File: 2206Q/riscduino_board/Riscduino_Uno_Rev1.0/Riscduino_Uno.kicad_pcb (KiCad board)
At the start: 2 copper layers, 68.8 x 53.6 mm, 80 parts, among them J1 USB_B_Micro, J10 Conn_01x01, J11 Conn_01x01, J2 ISP, J3 Conn_01x08_Pin, J4 Conn_01x06_Pin, J5 Conn_01x08_Pin, J6 Conn_01x10_Pin, J7 Conn_02x04_Odd_Even, J8 Conn_01x01, J9 Conn_01x01, SW1 4Pin Round Button SPST Straig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, U1 LM1117S-ADJ, U2 LM1117MP-3.3, U3 Riscduino, U4 CP2102N-Axx-xQFN28, U5 W25Q32JVSS, U6 W25Q32JVSS, U7 23LC1024-I/P, U8 MAX1232ESA+T, X1 ASE-10.000MHZ-LC-T

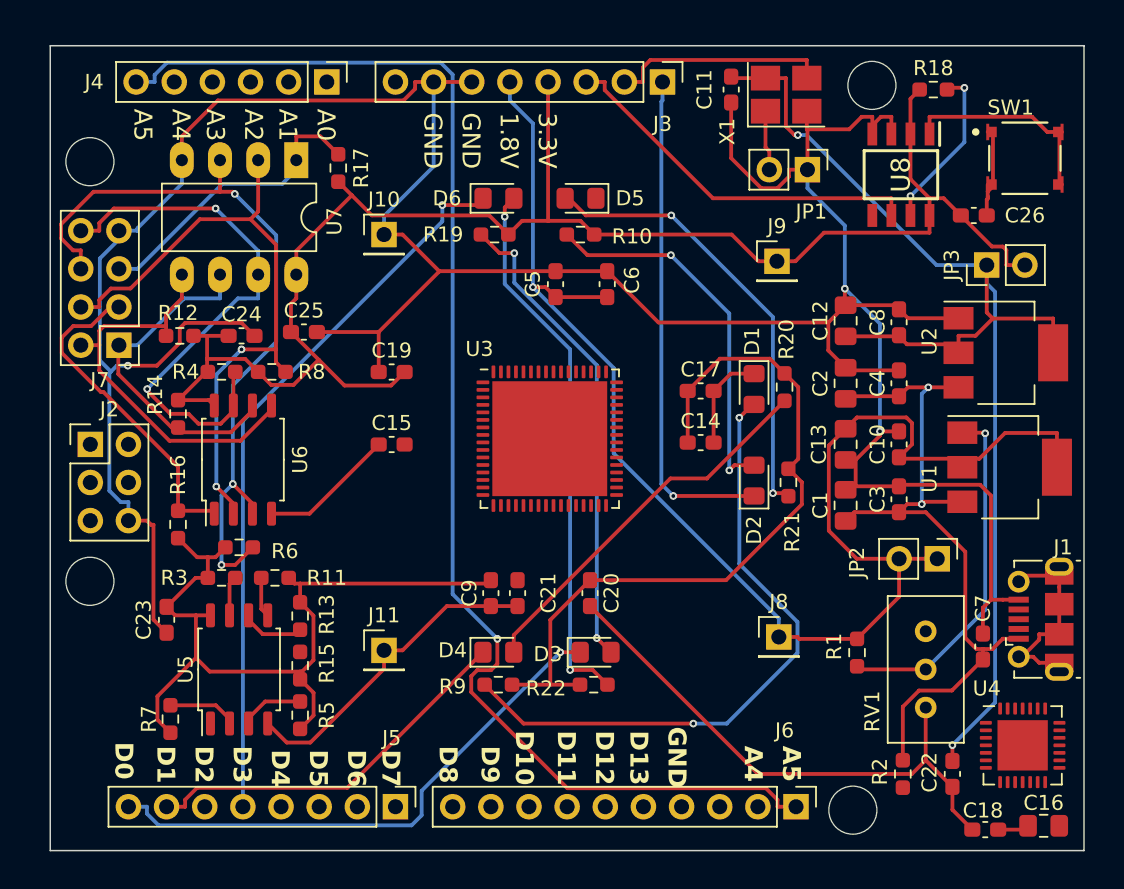
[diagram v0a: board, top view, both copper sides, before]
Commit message: 1.0.3 Update
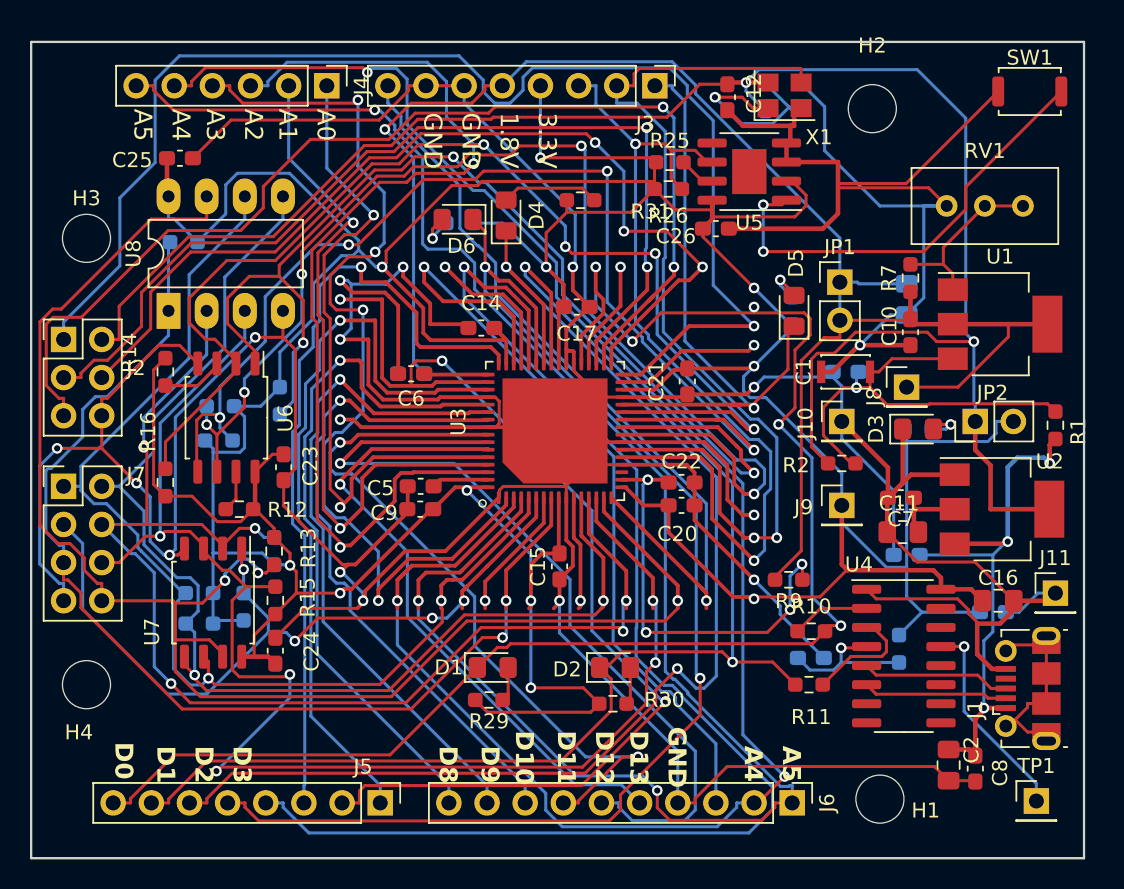
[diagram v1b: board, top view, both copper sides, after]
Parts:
- removed JP3: Jumper_2, Connector_PinHeader_2.54mm:PinHeader_1x02_P2.54mm_Vertical
- removed REF**: Riscduino_UNO_R0_WithMountingHoles, Riscduino.Library:Riscduino_UNO_R0_WithMountingHoles
- added H1: MountingHole, MountingHole:MountingHole_3.2mm_M3, F.Cu at (126.2, 99.8)
- added H2: MountingHole, MountingHole:MountingHole_3.2mm_M3, F.Cu at (125.7, 53.8)
- added H3: MountingHole, MountingHole:MountingHole_3.2mm_M3, F.Cu at (73.4, 62.5)
- added H4: MountingHole, MountingHole:MountingHole_3.2mm_M3, F.Cu at (73.4, 92.2)
- added R23: 10K, Resistor_SMD:R_0603_1608Metric_Pad0.98x0.95mm_HandSolder, B.Cu at (83.9, 87.0)
- added R24: 10K, Resistor_SMD:R_0603_1608Metric_Pad0.98x0.95mm_HandSolder, B.Cu at (79.9, 62.7)
- added R25: 10K, Resistor_SMD:R_0603_1608Metric_Pad0.98x0.95mm_HandSolder, F.Cu at (112.2, 57.4)
- added R26: 10K, Resistor_SMD:R_0603_1608Metric_Pad0.98x0.95mm_HandSolder, F.Cu at (112.1, 59.2)
- added R27: 470 Ohm, Resistor_SMD:R_0603_1608Metric_Pad0.98x0.95mm_HandSolder, B.Cu at (128.8, 75.2)
- added R28: 470 Ohm, Resistor_SMD:R_0603_1608Metric_Pad0.98x0.95mm_HandSolder, B.Cu at (120.4, 67.3)
- added R29: 470 Ohm, Resistor_SMD:R_0603_1608Metric_Pad0.98x0.95mm_HandSolder, F.Cu at (100.2, 93.2)
- added R30: 470 Ohm, Resistor_SMD:R_0603_1608Metric_Pad0.98x0.95mm_HandSolder, F.Cu at (108.5, 93.5)
- added R31: 470 Ohm, Resistor_SMD:R_0603_1608Metric_Pad0.98x0.95mm_HandSolder, F.Cu at (106.3, 59.9)
- added R32: 470 Ohm, Resistor_SMD:R_0603_1608Metric_Pad0.98x0.95mm_HandSolder, B.Cu at (98.3, 61.5)
- added TP1: TestPoint, Connector_PinHeader_2.54mm:PinHeader_1x01_P2.54mm_Vertical, F.Cu at (136.7, 99.9)
- C1: footprint Capacitor_SMD:C_0805_2012Metric_Pad1.18x1.45mm_HandSolder -> Button_Switch_SMD:SW_SPST_CK_KXT3
- C11: value 0.1uF -> 22uF; footprint Capacitor_SMD:C_0603_1608Metric_Pad1.08x0.95mm_HandSolder -> Capacitor_SMD:C_0805_2012Metric_Pad1.18x1.45mm_HandSolder
- C12: value 22uF -> 0.1uF; footprint Capacitor_SMD:C_0805_2012Metric_Pad1.18x1.45mm_HandSolder -> Capacitor_SMD:C_0603_1608Metric_Pad1.08x0.95mm_HandSolder
- C13, C18, C3, C4, R17, R18: moved to B.Cu
- C19: value 0.1uf -> 0.1uF; moved to B.Cu
- C22: value 0.1uF -> 0.1uf
- D1: value RED LED -> BLUE LED
- D3: value BLUE LED -> RED LED
- JP1: value Jumper_2_Open -> Jumper_2
- R1: value 470 Ohm -> DNI
- R10, R9: value 470 Ohm -> 0E
- R11, R2: value 10K -> 0E
- R19, R20, R21, R22: value 470 Ohm -> 10K; moved to B.Cu
- R3, R4, R8: value 10K -> 0E; moved to B.Cu
- R5, R6: value 10K -> DNI; moved to B.Cu
- R7: value 10K -> 470 Ohm
- SW1: footprint Switch_E-Switch_TL3315NF250Q:E-Switch-TL3315NF250Q-0-0-0 -> Button_Switch_SMD:SW_Push_SPST_NO_Alps_SKRK
- U3: footprint Package_DFN_QFN:QFN-64-1EP_9x9mm_P0.5mm_EP7.65x7.65mm -> Package_DFN_QFN:RISCDUINO_QFN-64-1EP_9x9mm_P0.5mm_EP7.65x7.65mm_NEW
- U4: value CP2102N-Axx-xQFN28 -> CH340C; footprint Package_DFN_QFN:QFN-28-1EP_5x5mm_P0.5mm_EP3.35x3.35mm -> Package_SO:SOIC-16_3.9x9.9mm_P1.27mm
- U5: value W25Q32JVSS -> MAX1232ESA+T; footprint Package_SO:SOIC-8_5.23x5.23mm_P1.27mm -> Package_SO:SOIC-8-1EP_3.9x4.9mm_P1.27mm_EP2.29x3mm
- U7: value 23LC1024-I/P -> W25Q32JVSS; footprint Package_DIP:DIP-8_W7.62mm_LongPads -> Package_SO:SOIC-8_5.23x5.23mm_P1.27mm
- U8: value MAX1232ESA+T -> 23LC1024-I/P; footprint MAX1232ESA+T:SOIC127P600X175-8N -> Package_DIP:DIP-8_W7.62mm_LongPads
- X1: footprint Oscillator:Oscillator_SMD_Abracon_ASE-4Pin_3.2x2.5mm_HandSoldering -> Crystal:Crystal_SMD_Abracon_ABM8G-4Pin_3.2x2.5mm
- moved R7 57.4 mm to (128.3, 65.1)
- moved R18 53.0 mm to (82.2, 75.9)
- moved R5 51.5 mm to (118.6, 53.1)
- moved U8 49.6 mm to (78.9, 67.3), turned to 90 degrees
- moved R6 47.9 mm to (120.9, 53.0), turned to 90 degrees
- moved U5 47.5 mm to (117.5, 58.0), turned to 180 degrees
- moved R8 45.6 mm to (127.5, 89.8), turned to 90 degrees
- moved J11 44.9 mm to (137.9, 86.1)
- moved R21 39.9 mm to (80.9, 86.1), turned to 180 degrees
- moved R20 37.6 mm to (82.3, 73.7), turned to 180 degrees
- moved R11 36.3 mm to (121.5, 92.2)
- moved C19 33.8 mm to (121.6, 90.4), turned to 180 degrees
- moved J10 32.9 mm to (123.7, 74.7)
- moved R19 32.5 mm to (80.9, 88.1), turned to 180 degrees
- moved C11 31.6 mm to (127.8, 82.0), turned to 180 degrees
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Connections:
- C1 pad 1: +5V -> Net-(U1-VI)
- C16 pad 1: +5V -> +3.3V
- C18 pad 1: +5V -> +3.3V
- C19 pad 2: +3.3V -> Net-(U4-V3)
- C20 pad 1: +3.3V -> GND
- C20 pad 2: GND -> +3.3V
- C21 pad 1: GND -> +3.3V
- C21 pad 2: +1V8 -> GND
- C22 pad 1: +3.3VP -> GND
- C22 pad 2: GND -> /vccd0
- C3 pad 1: +5V -> Net-(U1-VI)
- C5 pad 1: GND -> /vccd2
- C5 pad 2: +1V8 -> GND
- C6 pad 2: +1V8 -> /vccd1
- C7 pad 1: +5V -> +3.3VP
- C8 pad 1: +3.3VP -> +5V
- D1 pad 1: GND -> ardunio_d0
- D2 pad 1: gpio -> ardunio_d1
- D3 pad 1: ardunio_d0 -> GND
- D4 pad 1: ardunio_d1 -> ardunio_d2
- D5 pad 1: ardunio_d2 -> gpio
- JP1 pad 1: GND -> +1V8
- JP1 pad 2: Net-(JP1-B) -> +1V8
- JP2 pad 1: +1V8 -> +3.3VP
- JP2 pad 2: +1V8 -> +3.3V
- R1 pad 1: +1V8 -> +5V
- R1 pad 2: Net-(U1-ADJ) -> Net-(U1-VI)
- R10 pad 1: Net-(D2-A) -> Net-(U4-TXD)
- R10 pad 2: +3.3V -> ardunio_d0
- R11 pad 1: +3.3V -> Net-(U4-RXD)
- R11 pad 2: CARAVEL_FLASH_IO0 -> ardunio_d1
- R12 pad 2: USER_FLASH_IO0 -> CARAVEL_FLASH_IO3
- R13 pad 2: CARAVEL_FLASH_SCK -> USER_FLASH_IO3
- R14 pad 2: USER_FLASH_SCK -> CARAVEL_FLASH_IO2
- R15 pad 2: CARAVEL_FLASH_SSN -> USER_FLASH_IO2
- R16 pad 2: USER_FLASH_SSN -> CARAVEL_FLASH_IO1
- R17 pad 2: USER_SRAM_SSN -> USER_FLASH_IO1
- R18 pad 2: Net-(U8-~{ST}) -> CARAVEL_FLASH_IO0
- R19 pad 1: Net-(D3-A) -> +3.3V
- R19 pad 2: +3.3V -> USER_FLASH_IO0
- R2 pad 1: +5V -> +3.3VP
- R2 pad 2: Net-(U4-~{RST}) -> Net-(U1-VI)
- R20 pad 1: Net-(D4-A) -> +3.3V
- R20 pad 2: +3.3V -> CARAVEL_FLASH_SCK
- R21 pad 1: Net-(D5-A) -> +3.3V
- R21 pad 2: +3.3V -> USER_FLASH_SCK
- R22 pad 1: Net-(D6-A) -> +3.3V
- R22 pad 2: +3.3V -> CARAVEL_FLASH_SSN
- R3 pad 1: +3.3V -> +1V8
- R3 pad 2: CARAVEL_FLASH_IO3 -> /vccd2
- R4 pad 1: +3.3V -> +1V8
- R4 pad 2: USER_FLASH_IO3 -> /vccd1
- R5 pad 1: +3.3V -> +3.3VP
- R5 pad 2: CARAVEL_FLASH_IO2 -> Net-(X1-EN)
- R6 pad 1: +3.3V -> Net-(X1-EN)
- R6 pad 2: USER_FLASH_IO2 -> GND
- R7 pad 1: +3.3V -> +1V8
- R7 pad 2: CARAVEL_FLASH_IO1 -> Net-(U1-ADJ)
- R8 pad 1: +3.3V -> Net-(U4-V3)
- R8 pad 2: USER_FLASH_IO1 -> +3.3V
- R9 pad 1: Net-(D1-A) -> /vccd0
- R9 pad 2: +3.3V -> +1V8
- RV1 pad 1: unconnected-(RV1-Pad1) -> Net-(U1-ADJ)
- SW1 pad 2: Net-(U8-~{PB_RST}) -> Net-(U5-~{PB_RST})
- U1 pad 3: +5V -> Net-(U1-VI)
- U3 pad 18: +1V8 -> /vccd0
- U3 pad 49: +1V8 -> /vccd1
- U3 pad 63: +1V8 -> /vccd2
- U4 pad 1: unconnected-(U4-~{DCD}-Pad1) -> GND
- U4 pad 13: unconnected-(U4-CHREN-Pad13) -> Net-(U4-~{DTR})
- U4 pad 16: unconnected-(U4-~{WAKEUP}/GPIO.3-Pad16) -> +3.3V
- U4 pad 2: unconnected-(U4-~{RI}/CLK-Pad2) -> Net-(U4-TXD)
- U4 pad 3: GND -> Net-(U4-RXD)
- U4 pad 4: USB_D+ -> Net-(U4-V3)
- U4 pad 5: USB_D- -> USB_D+
- U4 pad 6: +3.3VP -> USB_D-
- U4 pad 7: +5V -> unconnected-(U4-NC-Pad7)
- U4 pad 8: +5V -> unconnected-(U4-NC-Pad8)
- U4 pad 9: Net-(U4-~{RST}) -> unconnected-(U4-~{CTS}-Pad9)
- U5 pad 1: CARAVEL_FLASH_SSN -> Net-(U5-~{PB_RST})
- U5 pad 2: CARAVEL_FLASH_IO1 -> +3.3V
- U5 pad 3: CARAVEL_FLASH_IO2 -> GND
- U5 pad 5: CARAVEL_FLASH_IO0 -> unconnected-(U5-RST-Pad5)
- U5 pad 6: CARAVEL_FLASH_SCK -> ~{RST}
- U5 pad 7: CARAVEL_FLASH_IO3 -> Net-(U5-~{ST})
- U6 pad 1: USER_FLASH_SSN -> CARAVEL_FLASH_SSN
- U6 pad 2: USER_FLASH_IO1 -> CARAVEL_FLASH_IO1
- U6 pad 3: USER_FLASH_IO2 -> CARAVEL_FLASH_IO2
- U6 pad 5: USER_FLASH_IO0 -> CARAVEL_FLASH_IO0
- U6 pad 6: USER_FLASH_SCK -> CARAVEL_FLASH_SCK
- U6 pad 7: USER_FLASH_IO3 -> CARAVEL_FLASH_IO3
- U7 pad 1: USER_SRAM_SSN -> USER_FLASH_SSN
- U8 pad 1: Net-(U8-~{PB_RST}) -> USER_SRAM_SSN
- U8 pad 2: +3.3V -> USER_FLASH_IO1
- U8 pad 3: GND -> USER_FLASH_IO2
- U8 pad 5: unconnected-(U8-RST-Pad5) -> USER_FLASH_IO0
- U8 pad 6: ~{RST} -> USER_FLASH_SCK
- U8 pad 7: Net-(U8-~{ST}) -> USER_FLASH_IO3
- X1 pad 1: Net-(JP1-B) -> Net-(X1-EN)
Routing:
- net GND: track 296.5 -> 463.6 mm, vias 3 -> 16
- net +3.3V: track 213.8 -> 346.0 mm, vias 0 -> 11
- net ardunio_a4: track 0.00 -> 123.2 mm, vias 0 -> 3
- net ardunio_d4: track 0.00 -> 89.4 mm, vias 0 -> 1
- net ISP_MISO: track 0.00 -> 87.6 mm, vias 0 -> 1
- net ardunio_d2: track 0.00 -> 83.3 mm, vias 0 -> 2
- net CARAVEL_FLASH_SCK: track 4.25 -> 81.5 mm, vias 0 -> 5
- net CARAVEL_FLASH_SSN: track 0.00 -> 75.6 mm, vias 0 -> 3
- net ISP_SSN: track 0.00 -> 74.4 mm, vias 0 -> 2
- net CARAVEL_FLASH_IO0: track 2.67 -> 75.7 mm, vias 0 -> 4
- net ardunio_d6: track 0.00 -> 72.7 mm, vias 0 -> 3
- net CARAVEL_FLASH_IO1: track 4.61 -> 77.3 mm, vias 0 -> 4
- net USER_FLASH_IO3: track 36.7 -> 104.2 mm, vias 2 -> 3
- net ardunio_a2: track 0.00 -> 67.1 mm, vias 0 -> 2
- net ardunio_d0: track 36.6 -> 102.6 mm, vias 1 -> 5
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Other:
- board size 68.8 x 53.6 mm -> 70.1 x 54.4 mm
- board text removed: "D4"
- board text removed: "D5"
- board text removed: "D6"
- board text removed: "D7"
